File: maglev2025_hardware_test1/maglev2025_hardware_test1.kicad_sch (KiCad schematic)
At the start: 5 parts, among them U1 STM32G474RBTx, U2 ICM-42688-P, U3 LIS3MDLTR, U4 AT8236

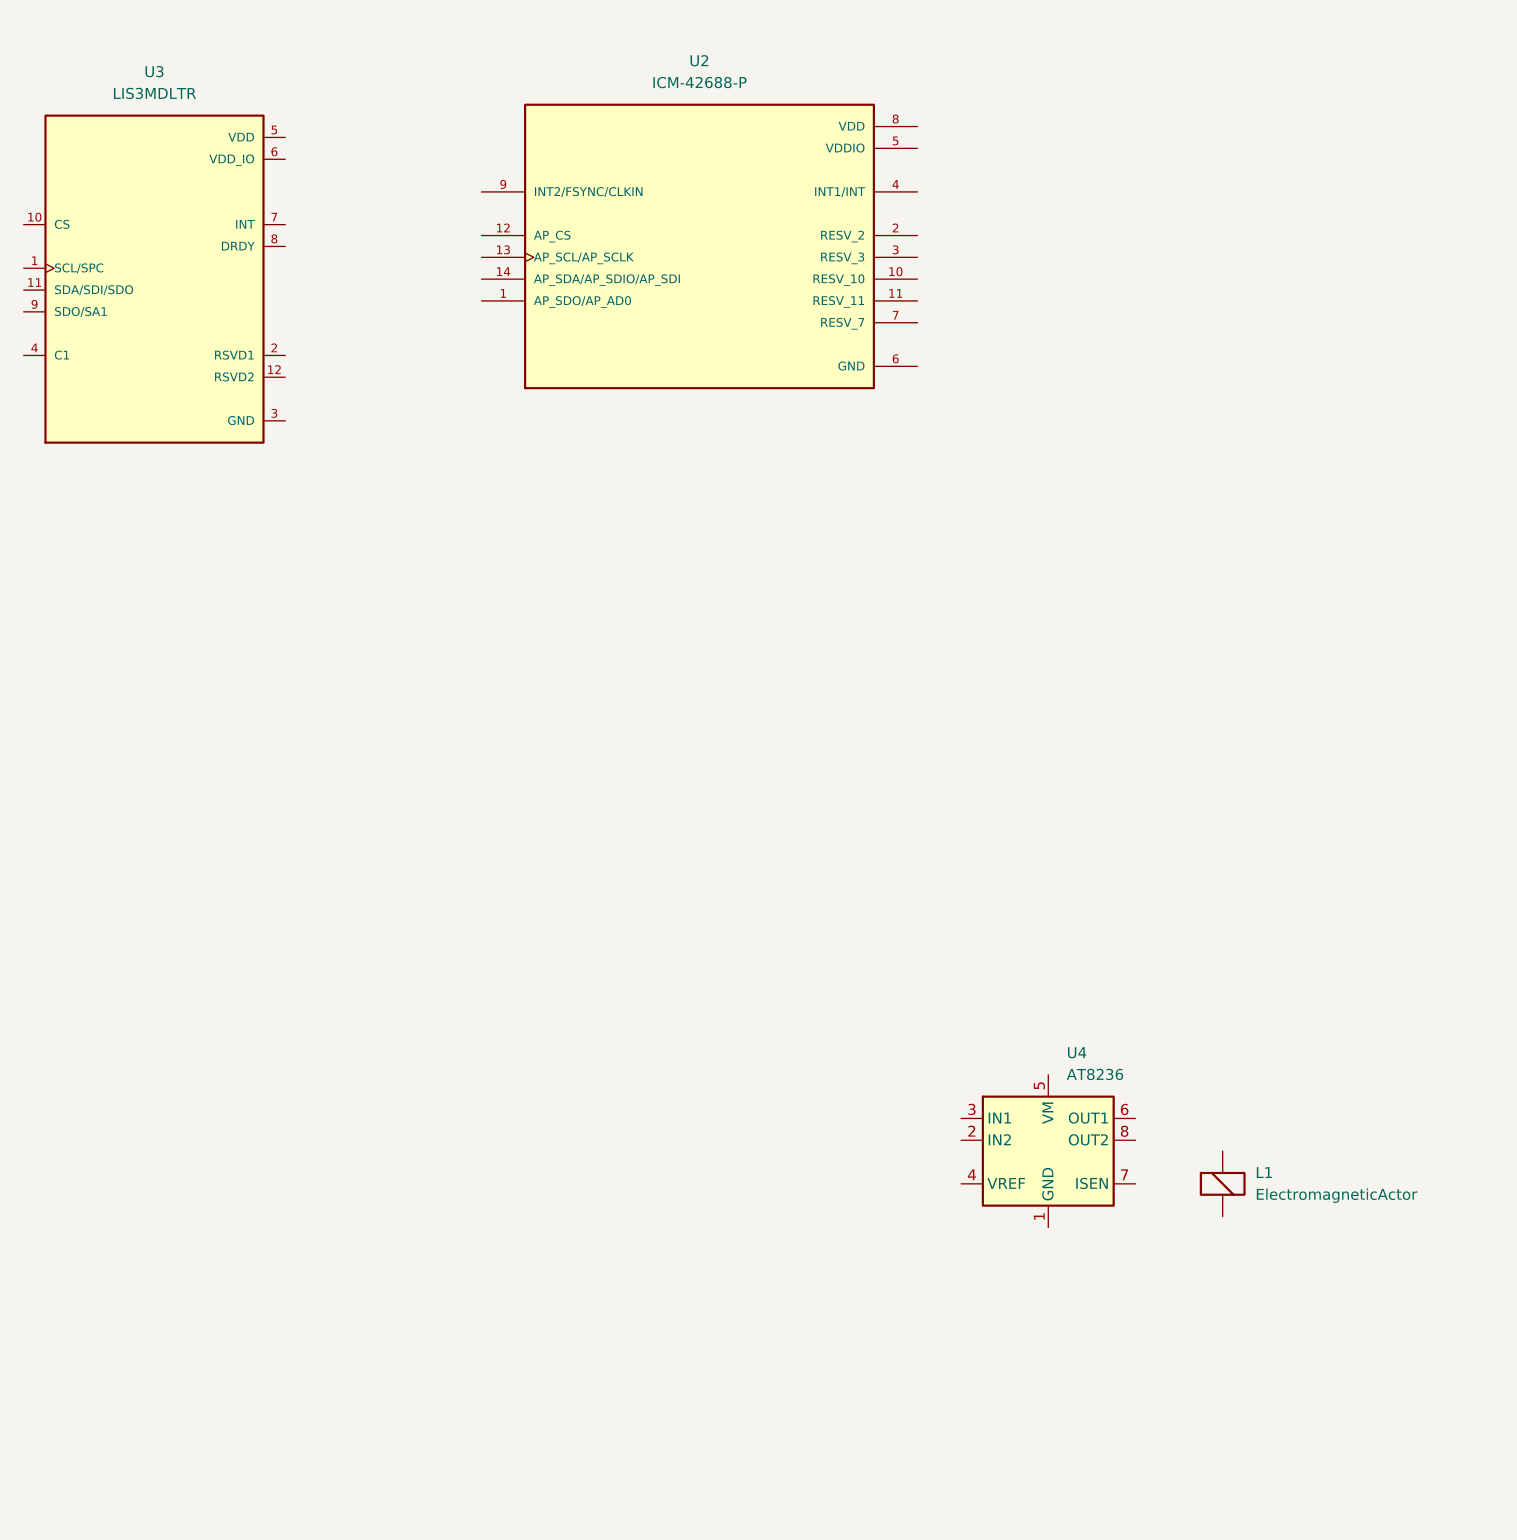
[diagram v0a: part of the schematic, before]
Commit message: update
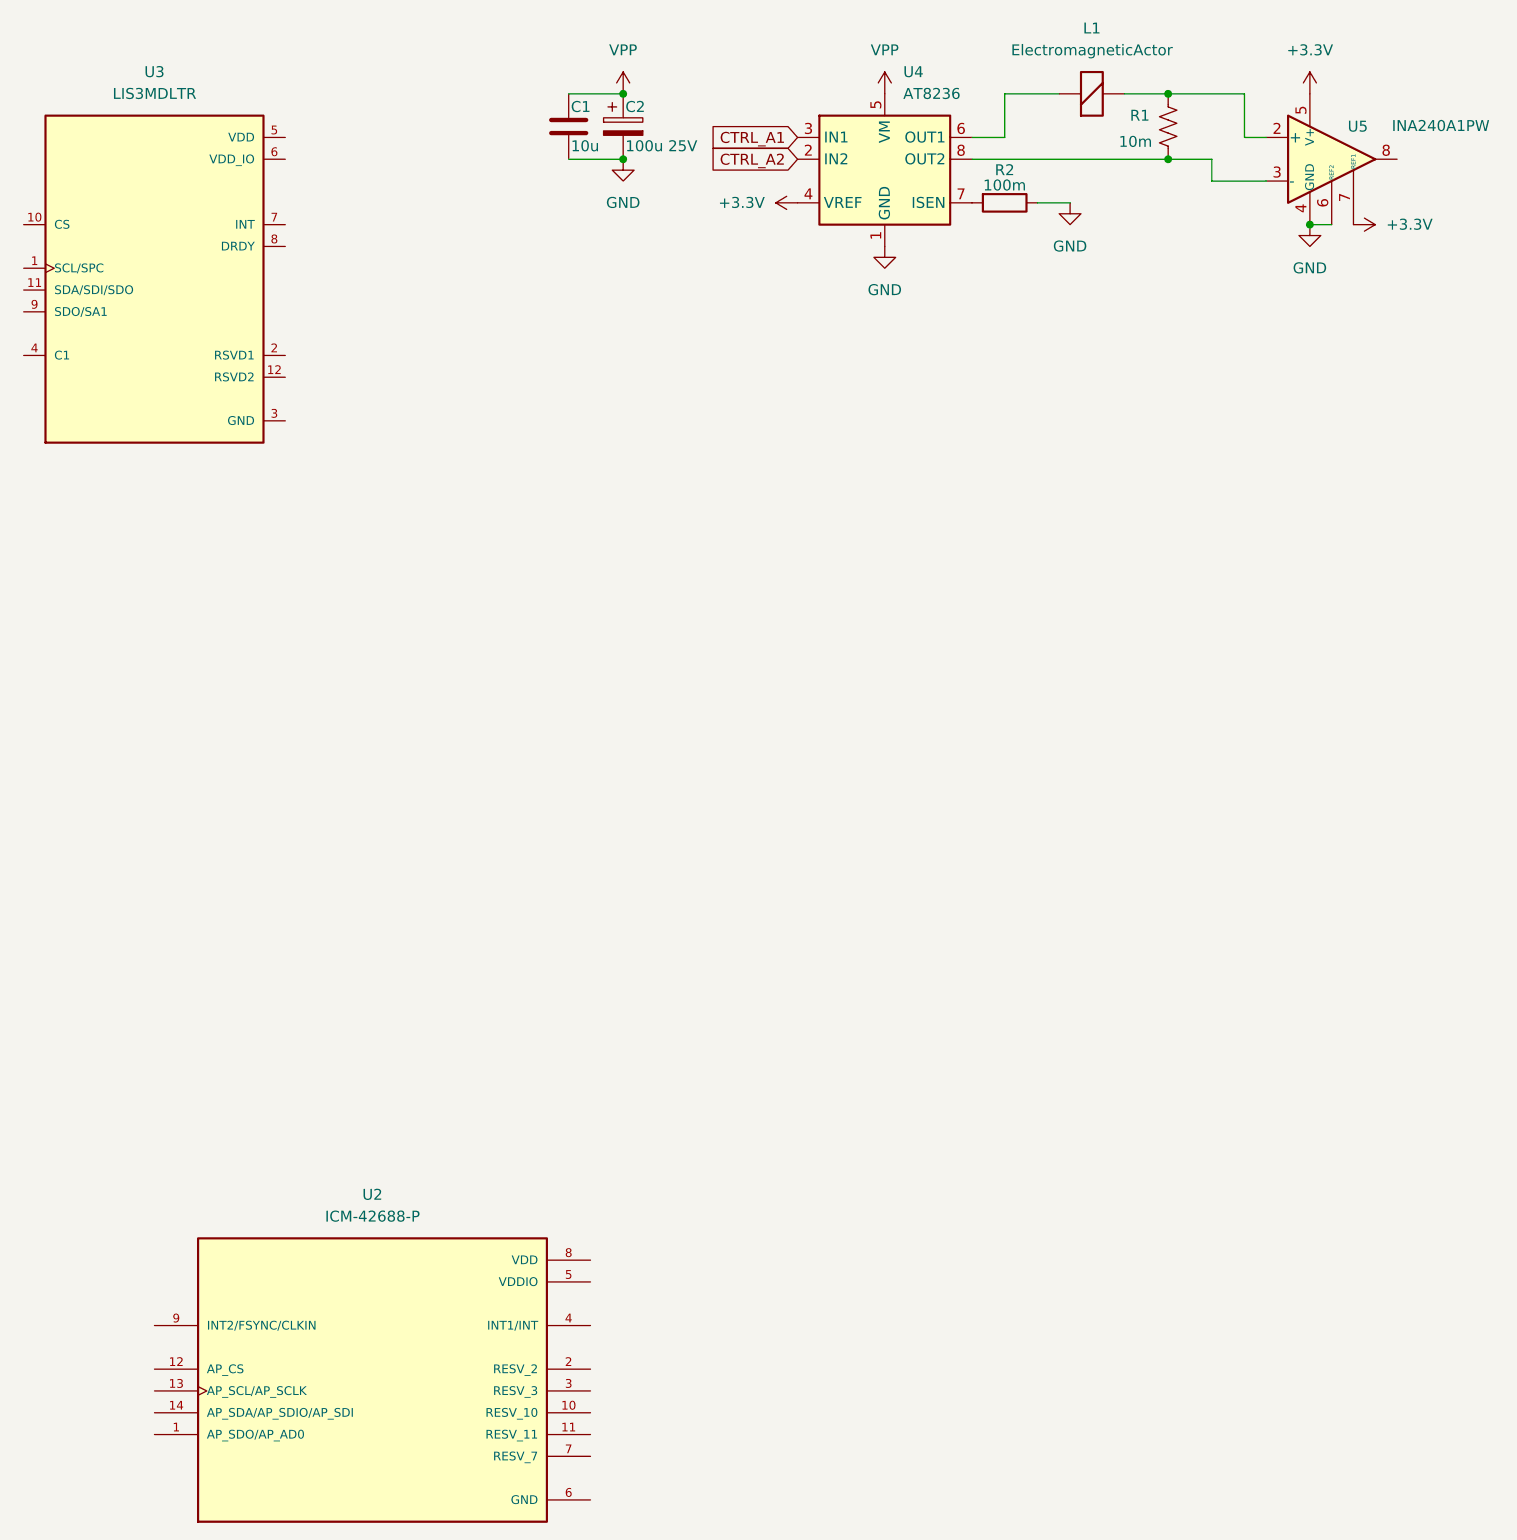
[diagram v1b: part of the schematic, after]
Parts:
- added C1: 10u, Capacitor_SMD:C_1206_3216Metric, symbol Device:C
- added C2: 100u 25V, Capacitor_THT:CP_Radial_D6.3mm_P2.50mm, symbol Device:C_Polarized
- added R1: 10m, Resistor_SMD:R_2512_6332Metric, symbol Device:R_US
- added R2: 100m, Resistor_SMD:R_2512_6332Metric, symbol Device:R
- added U5: INA240A1PW, Package_SO:TSSOP-8_4.4x3mm_P0.65mm, symbol Amplifier_Current:INA240A1PW
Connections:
- net at L1.1 (-): now also U4.6 (OUT1)
- net at L1.2 (+): now also R1.1, U5.2 (+)
- net GND: now reaches U4.1 (GND), U4.9 (GND)
- net GND: now also C1.2, C2.2, R2.1, U5.1 (GND), U5.4 (GND), U5.6 (REF2)
- net CTRL_A2: now reaches U4.2 (IN2)
- net CTRL_A1: now reaches U4.3 (IN1)
- net +3.3V: now reaches U4.4 (VREF)
- net +3.3V: now also U5.5 (V+), U5.7 (REF1)
- net VPP: now reaches U4.5 (VM)
- net VPP: now also C1.1, C2.1
- net at U4.7 (ISEN): now also R2.2
- net at U4.8 (OUT2): now also R1.2, U5.3 (-)
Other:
- moved on the sheet: L1, U2, U4

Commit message: schemetic and pin assignment
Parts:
- removed U2: ICM-42688-P, 0_RM2024:PQFN50P300X250X97-14N, symbol 0_RM2024:ICM-42688-P
- removed U3: LIS3MDLTR, 0_RM2024:XDCR_LIS3MDLTR, symbol 0_RM2024:LIS3MDLTR
- added C10, C9: 100u 16V, Capacitor_THT:CP_Radial_D6.3mm_P2.50mm, symbol Device:C_Polarized
- added C11: 10u, Capacitor_SMD:C_0603_1608Metric, symbol Device:C
- added C12, C13, C14, C15, C16, C17, C18, C19, C20, C23, C25, C27, C28, C31, C32, C33: 100n, Capacitor_SMD:C_0603_1608Metric, symbol Device:C
- added C21, C30, C40, C41: 100n, Capacitor_SMD:C_0603_1608Metric, symbol Device:C_Small
- added C22: 20p, Capacitor_SMD:C_0603_1608Metric, symbol Device:C_Small
- added C24, C26, C29: 10u, Capacitor_SMD:C_1206_3216Metric, symbol Device:C_Small
- added C3, C5, C6: 10u, Capacitor_SMD:C_1206_3216Metric, symbol Device:C
- added C36, C39, C78: 10u, Capacitor_SMD:C_0603_1608Metric, symbol Device:C_Small
- added C38: 10n, Capacitor_SMD:C_0603_1608Metric, symbol Device:C_Small
- added C4, C7, C8: 100u 25V, Capacitor_THT:CP_Radial_D6.3mm_P2.50mm, symbol Device:C_Polarized
- added D4: SMAJ12A, Diode_SMD:D_SMA, symbol Diode:SMAJ24A
- added D5: SMF5.0A, Diode_SMD:D_SMF, symbol Diode:SMAJ5.0A
- added F1: 1A, Fuse:Fuse_1206_3216Metric, symbol Device:Fuse
- added J20: PWRIn, Connector_AMASS:AMASS_XT30U-M_1x02_P5.0mm_Vertical, symbol Connector_Generic:Conn_01x02
- added J28: SWD, Connector_Molex:Molex_PicoBlade_53261-0471_1x04-1MP_P1.25mm_Horizontal, symbol Connector_Generic_MountingPin:Conn_01x04_MountingPin
- added L2, L3, L4: ElectromagneticActor, Inductor_SMD:L_APV_APH1030, symbol Device:ElectromagneticActor
- added L5: 6u8, Inductor_SMD:L_Sunlord_MWSA0402S, symbol Device:L
- added R10, R9: 10k, Resistor_SMD:R_0603_1608Metric, symbol Device:R
- added R11, R16: 33r, Resistor_SMD:R_0603_1608Metric, symbol Device:R
- added R12, R13, R14, R15: 33, Resistor_SMD:R_0603_1608Metric, symbol Device:R
- added R23: 53.6k, Resistor_SMD:R_0603_1608Metric, symbol Device:R_Small
- added R26: 10k, Resistor_SMD:R_0603_1608Metric, symbol Device:R_Small
- added R3, R5, R6: 100m, Resistor_SMD:R_2512_6332Metric, symbol Device:R
- added R4, R7, R8: 10m, Resistor_SMD:R_2512_6332Metric, symbol Device:R_US
- added RN1, RN2, RN3: 33x4, Resistor_SMD:R_Array_Convex_4x0603, symbol Device:R_Pack04
- added U10, U11, U7: INA240A1PW, Package_SO:TSSOP-8_4.4x3mm_P0.65mm, symbol Amplifier_Current:INA240A1PW
- added U12: RY8411, Package_TO_SOT_SMD:SOT-23-6, symbol RM24:SY8301
- added U13: RS3236, Package_TO_SOT_SMD:SOT-23-5, symbol Regulator_Linear:LDK130-12_SOT23_SOT353
- added U2: LIS3MDL, Package_LGA:LGA-12_2x2mm_P0.5mm, symbol Sensor_Magnetic:LIS3MDL
- added U6, U8, U9: AT8236, Package_SO:Texas_HTSOP-8-1EP_3.9x4.9mm_P1.27mm_EP2.95x4.9mm_Mask2.4x3.1mm_ThermalVias, symbol Driver_Motor:DRV8870DDA
- added Y1: 25MHz, Crystal:Crystal_SMD_3225-4Pin_3.2x2.5mm, symbol Device:Crystal_GND24
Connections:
- net +3.3V: now also U1.1 (VBAT), U1.16 (VDD), U1.29 (VDDA), U1.32 (VDD), U1.48 (VDD), U1.64 (VDD), C13.1, C14.1, C15.1, C16.1, C17.1, C18.1, C19.1, C32.1, C33.1, C39.1, C41.1, R9.1, U10.5 (V+), U10.7 (REF1), U11.5 (V+), U11.7 (REF1), U13.5 (OUT), U2.5 (Vdd), U2.6 (Vdd_IO), U6.4 (VREF), U7.5 (V+), U7.7 (REF1), U8.4 (VREF), U9.4 (VREF)
- net CTRL_A1: now also RN1.4 (R4.1)
- net CTRL_A2: now also RN1.3 (R3.1)
- net GND: now also U1.15 (VSS), U1.27 (VSSA), U1.31 (VSS), U1.47 (VSS), U1.63 (VSS), C10.2, C11.2, C12.2, C13.2, C14.2, C15.2, C16.2, C17.2, C18.2, C19.2, C20.1, C23.2, C24.2, C25.1, C26.2, C27.1, C28.1, C29.2, C3.2, C30.2, C31.1, C32.2, C33.2, C36.2, C38.2, C39.2, C4.2, C40.2, C41.2, C5.2, C6.2, C7.2, C78.2, C8.2, C9.2, D4.2 (A2), D5.2 (A2), J20.1 (Pin_1), J28.3 (Pin_3), J28.MP (MountPin), R10.2, R26.2, R3.1, R5.1, R6.1, U10.1 (GND), U10.4 (GND), U10.6 (REF2), U11.1 (GND), U11.4 (GND), U11.6 (REF2), U12.2 (GND), U13.2 (GND), U2.12 (GND), U2.2 (GND), U2.3 (GND), U6.1 (GND), U6.9 (GND), U7.1 (GND), U7.4 (GND), U7.6 (REF2), U8.1 (GND), U8.9 (GND), U9.1 (GND), U9.9 (GND), Y1.2, Y1.4
- net VPP: now also C10.1, C29.1, C3.1, C30.1, C4.1, C5.1, C6.1, C7.1, C8.1, D4.1 (A1), F1.2, U12.4 (EN), U12.5 (IN), U6.5 (VM), U8.5 (VM), U9.5 (VM)
- net ISENSE_A_MCU: now reaches U1.18 (PA4)
- net ISENSE_A_MCU: now also R12.1
- net ISENSE_B_MCU: now reaches U1.20 (PA6)
- net ISENSE_B_MCU: now also R13.1
- net ISENSE_C_MCU: now reaches U1.22 (PC4)
- net ISENSE_C_MCU: now also R14.1
- net ISENSE_D_MCU: now reaches U1.26 (PB2)
- net ISENSE_D_MCU: now also R15.1
- net VREF: now reaches U1.28 (VREF+)
- net VREF: now also C11.1, C12.1
- net MCU_C1: now reaches U1.34 (PB12)
- net MCU_C1: now also RN2.5 (R4.2)
- net MCU_C2: now reaches U1.35 (PB13)
- net MCU_C2: now also RN2.6 (R3.2)
- net MCU_D1: now reaches U1.36 (PB14)
- net MCU_D1: now also RN2.7 (R2.2)
- net MCU_D2: now reaches U1.37 (PB15)
- net MCU_D2: now also RN2.8 (R1.2)
- net MCU_A1: now reaches U1.42 (PA8)
- net MCU_A1: now also RN1.5 (R4.2)
- net MCU_A2: now reaches U1.43 (PA9)
- net MCU_A2: now also RN1.6 (R3.2)
- net MCU_B1: now reaches U1.44 (PA10)
- net MCU_B1: now also RN1.7 (R2.2)
- net MCU_B2: now reaches U1.45 (PA11)
- net MCU_B2: now also RN1.8 (R1.2)
- net at U1.5 (PF0): now also Y1.1
- net at U1.56 (PB3): now also RN3.5 (R4.2)
- net at U1.57 (PB4): now also RN3.6 (R3.2)
- net at U1.58 (PB5): now also RN3.7 (R2.2)
- net at U1.59 (PB6): now also RN3.8 (R1.2)
- net at U1.6 (PF1): now also Y1.3
- net at U1.60 (PB7): now also R11.1
- net BOOT0: now reaches U1.61 (PB8)
- net BOOT0: now also R10.1
- net at U1.62 (PB9): now also R16.1
- net NRST: now reaches U1.7 (PG10)
- net NRST: now also C20.2, R9.2
- net ISENSE_A: now reaches U5.8
- net ISENSE_A: now also C25.2, R12.2
- new net: L3.1 (-), U8.6 (OUT1)
- new net: L3.2 (+), R7.1, U10.2 (+)
- new net: C21.2, L5.1, U12.6 (LX)
- new net: F1.1, J20.2 (Pin_2)
- new net: C23.1, U2.4 (C1)
- new net: C22.2, R23.2, R26.1, U12.3 (FB)
- new net: L2.2 (+), R4.1, U7.2 (+)
- new net: R4.2, U6.8 (OUT2), U7.3 (-)
- new net: L4.2 (+), R8.1, U11.2 (+)
- new net: R8.2, U11.3 (-), U9.8 (OUT2)
- new net: R7.2, U10.3 (-), U8.8 (OUT2)
- new net: L4.1 (-), U9.6 (OUT1)
- new net: R6.2, U9.7 (ISEN)
- new net: C38.1, U13.4 (BP)
- new net: C21.1, U12.1 (BS)
- new net: R3.2, U6.7 (ISEN)
- new net: R5.2, U8.7 (ISEN)
- new net: L2.1 (-), U6.6 (OUT1)
- new net 3V3_SWD: C78.1, J28.4 (Pin_4)
- new net 5V: C22.1, C24.1, C26.1, C36.1, C40.1, C9.1, D5.1 (A1), L5.2, R23.1, U13.1 (IN), U13.3 (EN)
- new net CTRL_B1: RN1.2 (R2.1), U6.3 (IN1)
- new net CTRL_B2: RN1.1 (R1.1), U6.2 (IN2)
- new net CTRL_C1: RN2.4 (R4.1), U8.3 (IN1)
- new net CTRL_C2: RN2.3 (R3.1), U8.2 (IN2)
- new net CTRL_D1: RN2.2 (R2.1), U9.3 (IN1)
- new net CTRL_D2: RN2.1 (R1.1), U9.2 (IN2)
- new net ISENSE_B: C27.2, R13.2, U7.8
- new net ISENSE_C: C28.2, R14.2, U10.8
- new net ISENSE_D: C31.2, R15.2, U11.8
- new net LIS3_CS: R11.2, U2.10 (~{CS})
- new net LIS3_DRY: RN3.1 (R1.1), U2.8 (DRDY)
- new net LIS3_INT: R16.2, U2.7 (INT)
- new net SPI1_MISO: RN3.3 (R3.1), U2.9 (SDO/SA1)
- new net SPI1_MOSI: RN3.2 (R2.1), U2.11 (SDA/SDI/SDO)
- new net SPI1_SCK: RN3.4 (R4.1), U2.1 (SCL/SPC)
- new net SWCLK: J28.2 (Pin_2)
- new net SWDIO: J28.1 (Pin_1)
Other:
- note added: "12V IN"
- note added: "SWD"
- moved on the sheet: C1, C2, L1, R1, R2, U1, U4, U5
